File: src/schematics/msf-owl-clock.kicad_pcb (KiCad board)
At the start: 4 copper layers, 130.1 x 183.6 mm, 448 parts, among them Q101 NX6008NBKW, Q301 NX6008NBKW, Q501 NX6008NBKW, Q502 NX6008NBKW, Q503 NX6008NBKW, Q504 NX6008NBKW, Q505 NX6008NBKW, Q601 NX6008NBKW, Q602 BC847BS, Q603 BC847BS, U001 BC805M, U002 TSOP75338TT, U101 MP5016HGQH, U102 BQ24392RSER, U103 FUSB302BMPX, U104 TPS628512DRLR, U201 TPS7A2040PDQNR, U202 TPS7A2036PDBVR, U203 MCP6499, U204 MCP6499, U205 74HC595BQ, U206 TMUX1511RSV, U207 TMUX1511RSV, U301 PIC32CX1025SG41100-I/E5X, U302 AP22653AW6, U401 AP22653AW6, U402 MCP6486U, U403 IS31AP4991A-SLS2, U501 TPS7A2028PDBVR, U502 DPS310XTSA1, U503 HDC3022, U504 VL6180V1NR1, U601 TMUX1574RSV, U602 TMUX1574RSV, U603 TMUX1574RSV

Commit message: Added tie-wrap holes for the talons, along with a 3D model of the tie-wraps.
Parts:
- added TALON-LEFT: talon, msf-owl-clock:talon, F.Cu at (124.0, 181.5)
- added TALON-RIGHT: talon, msf-owl-clock:talon, F.Cu at (76.0, 181.5)
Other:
- board text removed: "TODO: PLACE THE HOLES (2x (3x 2.5mm TIE-WRAPS)) SLIGHTLY BEHIND THE FERRITE BAR, OR LEVEL WITH THE TOP OF ? WHICH ONE WILL FIT THE CURVE OF THE TIE-WRAPS BETTER AND LOOK BETTER ?"
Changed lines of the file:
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@@
     )
   )
+  (footprint "msf-owl-clock:talon" (layer "F.Cu")
+    (at 124 181.5)
+    (descr "Cut-Outs for Tie-Wraps - Serves as Talons")
+    (tags "owl-msf owl msf tie-wrap tie-wraps tiewrap tiewraps tie wrap wraps talon talons")
+    (attr through_hole board_only exclude_from_pos_files exclude_from_bom allow_missing_courtyard)
+    (fp_text reference "TALON-LEFT" (at 0 -2.4) (layer "F.SilkS") hide
+        (effects (font (size 1 1) (thickness 0.15)))
+    )
+    (fp_text value "talon" (at 0 2.2) (layer "F.Fab")
+        (effects (font (size 1 1) (thickness 0.15)))
+    )
+    (fp_text user "${REFERENCE}" (at 0 0) (layer "F.Fab")
+        (effects (font (size 0.98 0.98) (thickness 0.15)))
+    )
+    (pad "" np_thru_hole oval (at -7.5 -6.125) (size 3.75 1.25) (drill oval 3.75 1.25) (layers "F&B.Cu" "*.Mask"))
+    (pad "" np_thru_hole oval (at -7.5 6.125) (size 3.75 1.25) (drill oval 3.75 1.25) (layers "F&B.Cu" "*.Mask"))
+    (pad "" np_thru_hole oval (at 0 -6.125) (size 3.75 1.25) (drill oval 3.75 1.25) (layers "F&B.Cu" "*.Mask"))
+    (pad "" np_thru_hole oval (at 0 6.125) (size 3.75 1.25) (drill oval 3.75 1.25) (layers "F&B.Cu" "*.Mask"))
+    (pad "" np_thru_hole oval (at 7.5 -6.125) (size 3.75 1.25) (drill oval 3.75 1.25) (layers "F&B.Cu" "*.Mask"))
+    (pad "" np_thru_hole oval (at 7.5 6.125) (size 3.75 1.25) (drill oval 3.75 1.25) (layers "F&B.Cu" "*.Mask"))
+    (model "${KIPRJMOD}/msf-owl-clock.pretty/talon.step"
+      (offset (xyz -7.5 0 2.6))
+      (scale (xyz 1 1 1))
+      (rotate (xyz 90 0 0))
+    )
+  )
   (footprint "restall-generic-capacitors:unpolarised-nominal-0805-2012" (layer "F.Cu")
     (at 335.81 102.42)
@@
     )
   )
+  (footprint "msf-owl-clock:talon" (layer "F.Cu")
+    (at 76 181.5)
+    (descr "Cut-Outs for Tie-Wraps - Serves as Talons")
+    (tags "owl-msf owl msf tie-wrap tie-wraps tiewrap tiewraps tie wrap wraps talon talons")
+    (attr through_hole board_only exclude_from_pos_files exclude_from_bom allow_missing_courtyard)
+    (fp_text reference "TALON-RIGHT" (at 0 -2.4) (layer "F.SilkS") hide
+        (effects (font (size 1 1) (thickness 0.15)))
+    )
+    (fp_text value "talon" (at 0 2.2) (layer "F.Fab")
+        (effects (font (size 1 1) (thickness 0.15)))
+    )
+    (fp_text user "${REFERENCE}" (at 0 0) (layer "F.Fab")
+        (effects (font (size 0.98 0.98) (thickness 0.15)))
+    )
+    (pad "" np_thru_hole oval (at -7.5 -6.125) (size 3.75 1.25) (drill oval 3.75 1.25) (layers "F&B.Cu" "*.Mask"))
+    (pad "" np_thru_hole oval (at -7.5 6.125) (size 3.75 1.25) (drill oval 3.75 1.25) (layers "F&B.Cu" "*.Mask"))
+    (pad "" np_thru_hole oval (at 0 -6.125) (size 3.75 1.25) (drill oval 3.75 1.25) (layers "F&B.Cu" "*.Mask"))
+    (pad "" np_thru_hole oval (at 0 6.125) (size 3.75 1.25) (drill oval 3.75 1.25) (layers "F&B.Cu" "*.Mask"))
+    (pad "" np_thru_hole oval (at 7.5 -6.125) (size 3.75 1.25) (drill oval 3.75 1.25) (layers "F&B.Cu" "*.Mask"))
+    (pad "" np_thru_hole oval (at 7.5 6.125) (size 3.75 1.25) (drill oval 3.75 1.25) (layers "F&B.Cu" "*.Mask"))
+    (model "${KIPRJMOD}/msf-owl-clock.pretty/talon.step"
+      (offset (xyz -7.5 0 2.6))
+      (scale (xyz 1 1 1))
+      (rotate (xyz 90 0 0))
+    )
+  )
   (footprint "restall-generic-resistors:nominal-0402-1005" (layer "F.Cu")
     (at 336.41 128.9)
@@
   (gr_line locked (start 46.438013 147.054717) (end 45.431775 145.916333)
     (stroke (width 0.2) (type solid)) (layer "Edge.Cuts"))
-  (gr_text "TODO: PLACE THE HOLES (2x (3x 2.5mm TIE-WRAPS)) SLIGHTLY BEHIND THE FERRITE BAR, OR LEVEL WITH THE TOP OF ?  WHICH ONE WILL FIT THE CURVE OF THE TIE-WRAPS BETTER AND LOOK BETTER ?" (at 100 178) (layer "Cmts.User")
-    (effects (font (size 1 1) (thickness 0.15)))
-  )
   (gr_text "PCB Capabilities:\nhttps://jlcpcb.com/capabilities/pcb-capabilities\n\nTooling Holes:\nhttps://jlcpcb.com/help/article/47-How-to-add-tooling-holes-for-PCB-assembly-order" (at 199.9 22) (layer "F.Fab")
     (effects (font (size 1 1) (thickness 0.15)) (justify left bottom))

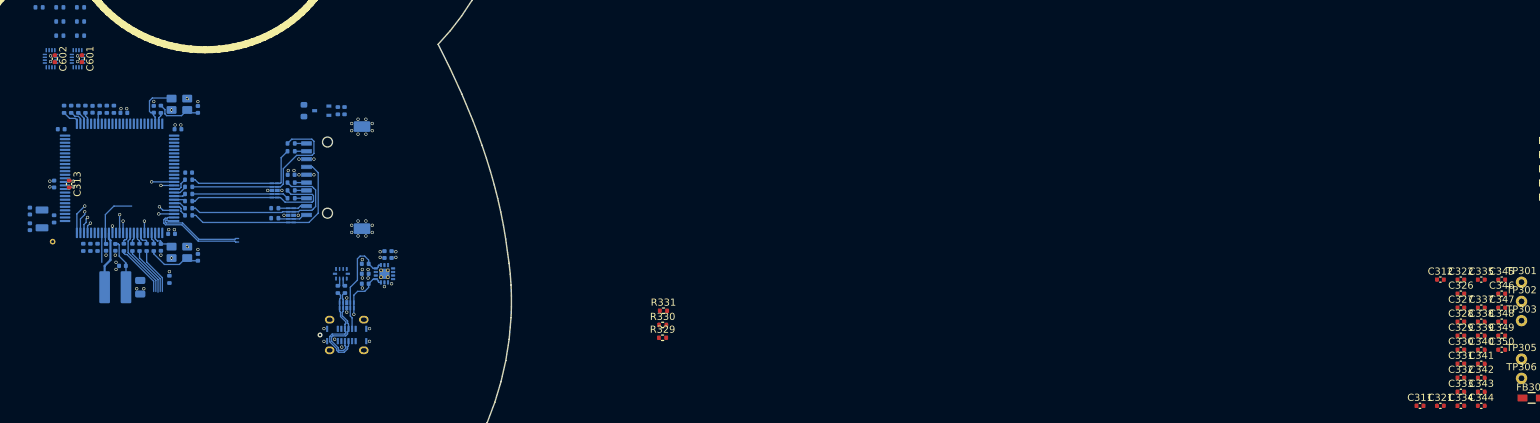
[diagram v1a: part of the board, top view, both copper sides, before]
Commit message: PCB routing.
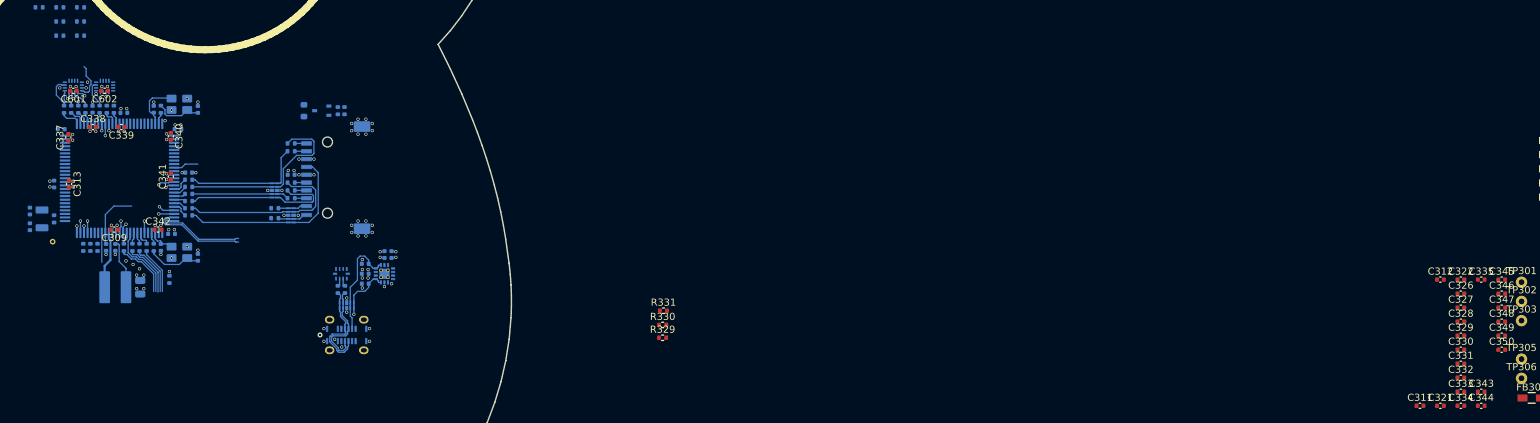
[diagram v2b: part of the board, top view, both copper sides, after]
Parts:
- C309: moved to F.Cu
- moved C337 199.9 mm to (102.8, 94.2), turned to 90 degrees
- moved C338 196.9 mm to (106.2, 92.8)
- moved C339 193.3 mm to (110.2, 92.8), turned to 180 degrees
- moved C342 187.1 mm to (115.4, 107.2)
- moved C340 186.5 mm to (117.2, 94.1), turned to -90 degrees
- moved C341 186.0 mm to (117.2, 99.8), turned to 90 degrees
- moved U602 8.54 mm to (107.9, 87.1), turned to 90 degrees
- moved C602 8.32 mm to (107.9, 87.7), turned to 180 degrees
- moved C309 5.23 mm to (109.2, 107.2)
- moved C601 4.67 mm to (103.5, 87.7), turned to 180 degrees
- moved U601 3.94 mm to (103.5, 87.1), turned to 90 degrees
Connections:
- R604 pad 1: /6-tft-driver/TFT1.L_{IO3} -> /6-tft-driver/TFT1.L_{SDIN}
- R605 pad 1: /6-tft-driver/TFT0.L_{IO3} -> /6-tft-driver/TFT0.L_{SDIN}
- R606 pad 1: /6-tft-driver/TFT1.L_{SCLK} -> /6-tft-driver/TFT1.L_{IO1}
- R607 pad 1: /6-tft-driver/TFT0.L_{SCLK} -> /6-tft-driver/TFT0.L_{IO1}
- R608 pad 1: /6-tft-driver/TFT1.L_{SDIN} -> /6-tft-driver/TFT1.L_{IO3}
- R609 pad 1: /6-tft-driver/TFT0.L_{SDIN} -> /6-tft-driver/TFT0.L_{IO3}
- R612 pad 1: /6-tft-driver/TFT1.L_{IO1} -> /6-tft-driver/TFT1.L_{SCLK}
- R613 pad 1: /6-tft-driver/TFT0.L_{IO1} -> /6-tft-driver/TFT0.L_{SCLK}
- U601 pad 1: /6-tft-driver/TFT1.L_{SDIN} -> /6-tft-driver/TFT1.L_{IO3}
- U601 pad 16: /6-tft-driver/TFT0.L_{SDIN} -> /6-tft-driver/TFT0.L_{IO3}
- U601 pad 2: /3-mcu-core/DATA0 -> /3-mcu-core/DATA3
- U601 pad 3: /6-tft-driver/TFT0.L_{SCLK} -> /6-tft-driver/TFT0.L_{IO1}
- U601 pad 4: /6-tft-driver/TFT1.L_{SCLK} -> /6-tft-driver/TFT1.L_{IO1}
- U601 pad 5: /3-mcu-core/SCK -> /3-mcu-core/DATA1
- U601 pad 7: /3-mcu-core/DATA3 -> /3-mcu-core/DATA0
- U601 pad 8: /6-tft-driver/TFT1.L_{IO3} -> /6-tft-driver/TFT1.L_{SDIN}
- U601 pad 9: /6-tft-driver/TFT0.L_{IO3} -> /6-tft-driver/TFT0.L_{SDIN}
- U602 pad 3: /6-tft-driver/TFT0.L_{IO1} -> GND
- U602 pad 4: /6-tft-driver/TFT1.L_{IO1} -> GND
- U602 pad 5: /3-mcu-core/DATA1 -> GND
- U602 pad 7: GND -> /3-mcu-core/SCK
- U602 pad 8: GND -> /6-tft-driver/TFT1.L_{SCLK}
- U602 pad 9: GND -> /6-tft-driver/TFT0.L_{SCLK}
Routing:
- net /6-tft-driver/TFT0.L_{IO3}: track 0.00 -> 5.15 mm
- net /3-mcu-core/DATA0: track 0.00 -> 4.47 mm
- net /3-mcu-core/SCK: track 0.00 -> 3.77 mm
- net Net-(U301-PC20): track 0.00 -> 3.54 mm
- net /3-mcu-core/~{HMD_ALERT}: track 4.22 -> 0.96 mm
- net /3-mcu-core/DATA1: track 0.00 -> 2.87 mm
- net /3-mcu-core/DATA3: track 0.00 -> 2.75 mm
- net Net-(U301-PB14): track 0.00 -> 2.15 mm
- net /3-mcu-core/TFT_TEAR0: track 0.00 -> 1.66 mm, vias 0 -> 1
- net Net-(U301-PB15): track 0.00 -> 1.65 mm
- net /3-mcu-core/~{BAR_INT}: track 3.21 -> 1.66 mm
- net /3-mcu-core/PRX_GPIO0: track 2.37 -> 0.96 mm
- net /6-tft-driver/TFT1.L_{IO3}: track 0.00 -> 1.37 mm, vias 0 -> 1
- net /6-tft-driver/TFT1.L_{IO1}: track 0.00 -> 0.98 mm, vias 0 -> 1
- net /6-tft-driver/TFT0.L_{IO1}: track 0.00 -> 0.98 mm, vias 0 -> 1
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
